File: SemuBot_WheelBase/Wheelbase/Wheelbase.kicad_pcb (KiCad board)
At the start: 2 copper layers, 100 x 80 mm, 120 parts, among them IC1 DRV8353FSRTAR, IC2 DRV8353FSRTAR, IC3 DRV8353FSRTAR, J1 10155435-00011LF, J10 B5B-XH-A_LF__SN_, J11 B5B-XH-A_LF__SN_, J12 B5B-XH-A_LF__SN_, J13 MTSW-104-09-L-S-400, J14 XT30PW-M, J15 MTSW-104-09-L-S-400, J2 MTSW-102-09-L-S-400, J3 MR30PW-M, J4 B5B-XH-A_LF__SN_, J5 B5B-XH-A_LF__SN_, J6 B5B-XH-A_LF__SN_, J7 MR30PW-M, J8 MR30PW-M, J9 DS1013-10SSIB1, Q1 AON7262E, Q10 AON7262E, Q11 AON7262E, Q12 AON7262E, Q13 AON7262E, Q14 AON7262E, Q15 AON7262E, Q19 AON7262E, Q2 AON7262E, Q20 AON7262E, Q21 AON7262E, Q3 AON7262E, Q4 AON7262E, Q5 AON7262E, Q6 AON7262E, Q7 AON7262E, Q8 AON7262E, Q9 AON7262E, U1 STM32F303RET6, U5 RT9013-33GB, Y2 X322516MLB4SI

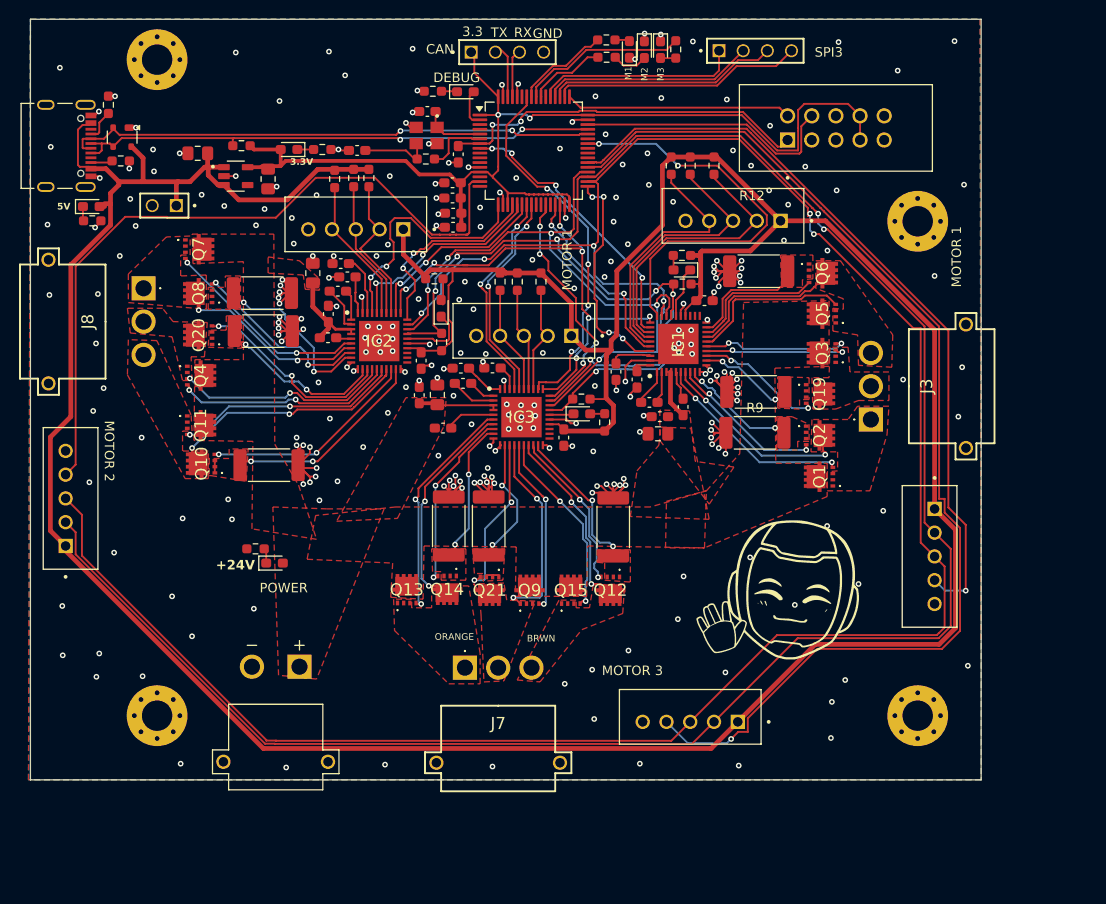
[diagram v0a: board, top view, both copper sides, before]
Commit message: Current sensing
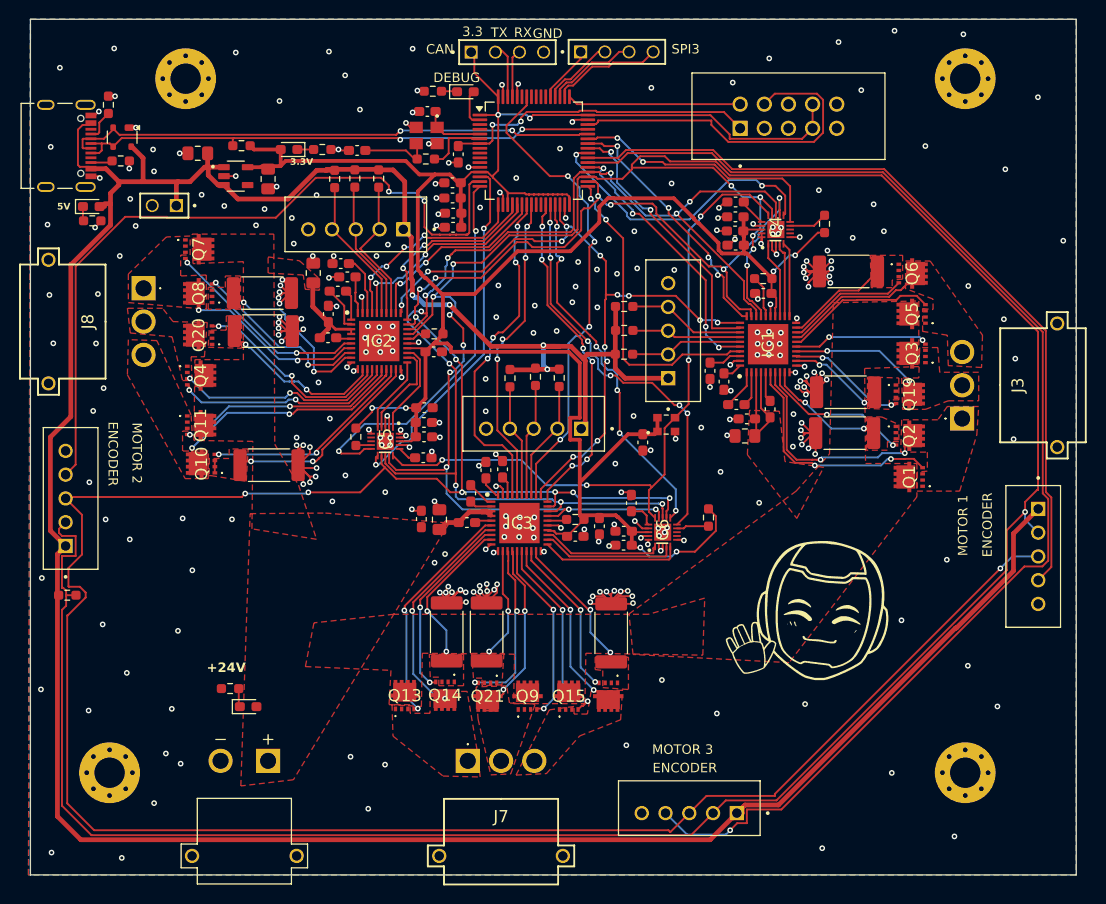
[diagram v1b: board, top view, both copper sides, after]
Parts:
- removed D10, D11, D12: red, LED_SMD:LED_0603_1608Metric_Pad1.05x0.95mm_HandSolder
- removed D4, D5, D6: LED, LED_SMD:LED_0603_1608Metric_Pad1.05x0.95mm_HandSolder
- removed the R21 at (162.3, 64.8)
- removed the R22 at (169.6, 63.9)
- removed R23, R24, R25: 3.3K, Resistor_SMD:R_0603_1608Metric_Pad0.98x0.95mm_HandSolder
- removed the R3 at (144.9, 94.7)
- added C16: 220nF, Capacitor_SMD:C_0603_1608Metric_Pad1.08x0.95mm_HandSolder, F.Cu at (175.8, 80.0)
- added C22: 220nF, Capacitor_SMD:C_0603_1608Metric_Pad1.08x0.95mm_HandSolder, F.Cu at (143.0, 106.9)
- added C34: 220nF, Capacitor_SMD:C_0603_1608Metric_Pad1.08x0.95mm_HandSolder, F.Cu at (164.9, 111.6)
- added C35: 100nF, Capacitor_SMD:C_0603_1608Metric_Pad1.08x0.95mm_HandSolder, F.Cu at (175.9, 84.5)
- added C36: 100nF, Capacitor_SMD:C_0603_1608Metric_Pad1.08x0.95mm_HandSolder, F.Cu at (143.1, 104.7)
- added C37: 100nF, Capacitor_SMD:C_0603_1608Metric_Pad1.08x0.95mm_HandSolder, F.Cu at (161.5, 114.1)
- added C38: 100nF, Capacitor_SMD:C_0603_1608Metric_Pad1.08x0.95mm_HandSolder, F.Cu at (175.8, 81.5)
- added C39: 100nF, Capacitor_SMD:C_0603_1608Metric_Pad1.08x0.95mm_HandSolder, F.Cu at (143.1, 103.2)
- added C40: 100nF, Capacitor_SMD:C_0603_1608Metric_Pad1.08x0.95mm_HandSolder, F.Cu at (164.1, 114.6)
- added C50: 100nF, Capacitor_SMD:C_0603_1608Metric_Pad1.08x0.95mm_HandSolder, F.Cu at (166.1, 105.3)
- added C51: 100nF, Capacitor_SMD:C_0603_1608Metric_Pad1.08x0.95mm_HandSolder, F.Cu at (175.8, 83.0)
- added C52: 100nF, Capacitor_SMD:C_0603_1608Metric_Pad1.08x0.95mm_HandSolder, F.Cu at (143.1, 101.6)
- added C53: 100nF, Capacitor_SMD:C_0603_1608Metric_Pad1.08x0.95mm_HandSolder, F.Cu at (164.1, 116.1)
- added IC4: ADS131M03IRUKT, ADS131M:QFN40P300X300X80-21N-D, F.Cu at (180.1, 82.9)
- added IC5: ADS131M03IRUKT, ADS131M:QFN40P300X300X80-21N-D, F.Cu at (139.0, 105.1)
- added IC6: ADS131M03IRUKT, ADS131M:QFN40P300X300X80-21N-D, F.Cu at (168.2, 114.7)
- added R32: 1.5K, Resistor_SMD:R_0603_1608Metric_Pad0.98x0.95mm_HandSolder, F.Cu at (164.1, 93.5)
- added R33: 1.5K, Resistor_SMD:R_0603_1608Metric_Pad0.98x0.95mm_HandSolder, F.Cu at (135.8, 77.5)
- added R34: 1.5K, Resistor_SMD:R_0603_1608Metric_Pad0.98x0.95mm_HandSolder, F.Cu at (154.8, 98.4)
- added R45: 3.3K, Resistor_SMD:R_0603_1608Metric_Pad0.98x0.95mm_HandSolder, F.Cu at (105.6, 121.3)
- added Y1: ECS-2520MVLC-081.92-CN-TR, ECS-2520:OSC_ECS-2520MVLC-081.92-CN-TR, F.Cu at (168.6, 103.4)
- moved H4 113.4 mm to (200.0, 140.0)
- moved H2 85.2 mm to (110.0, 140.0)
- moved H1 67.1 mm to (118.0, 67.0)
- moved R22 31.9 mm to (173.0, 113.2)
- moved R21 27.2 mm to (135.9, 104.7)
- moved R35 20.4 mm to (164.1, 96.0), turned to 180 degrees
- moved R29 17.6 mm to (164.1, 91.0), turned to 180 degrees
- moved H3 15.8 mm to (200.0, 67.0)
- moved R3 15.4 mm to (185.2, 82.3), turned to -90 degrees
- moved D7 15.4 mm to (124.6, 133.1)
- moved R18 14.9 mm to (122.7, 131.2)
- moved J15 14.6 mm to (163.4, 64.2)
- moved J4 13.6 mm to (169.3, 93.5), turned to -90 degrees
- moved C33 13.1 mm to (144.7, 113.4)
- moved C23 13.0 mm to (142.8, 113.3)
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- renumbered R33 to R21, R34 to R22, R32 to R3
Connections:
- C18 pad 1: +5V -> +3.3V
- C24 pad 1: +5V -> +3.3V
- C6 pad 1: +5V -> +3.3V
- IC1 pad 21: unconnected-(IC1-SOC-Pad21) -> /Motor_1/SOC
- IC1 pad 22: unconnected-(IC1-SOB-Pad22) -> /Motor_1/SOB
- IC1 pad 23: unconnected-(IC1-SOA-Pad23) -> /Motor_1/SOA
- IC1 pad 24: +5V -> +3.3V
- IC1 pad 26: Net-(D4-K) -> Net-(IC1-NFAULT)
- IC2 pad 21: unconnected-(IC2-SOC-Pad21) -> /Motor_2/SOC
- IC2 pad 22: unconnected-(IC2-SOB-Pad22) -> /Motor_2/SOB
- IC2 pad 23: unconnected-(IC2-SOA-Pad23) -> /Motor_2/SOA
- IC2 pad 24: +5V -> +3.3V
- IC2 pad 26: Net-(D5-K) -> Net-(IC2-NFAULT)
- IC3 pad 21: unconnected-(IC3-SOC-Pad21) -> /Motor_3/SOC
- IC3 pad 22: unconnected-(IC3-SOB-Pad22) -> /Motor_3/SOB
- IC3 pad 23: unconnected-(IC3-SOA-Pad23) -> /Motor_3/SOA
- IC3 pad 24: +5V -> +3.3V
- IC3 pad 26: Net-(D6-K) -> Net-(IC3-NFAULT)
- J4 pad 2: /Motor_1/HAL_1 -> /Motor_1/HAL_3
- J4 pad 4: /Motor_1/HAL_3 -> /Motor_1/HAL_1
- R21 pad 1: /Motor_2/HAL_2 -> Net-(IC5-~{SYNC_}/_~{RESET})
- R21 pad 2: +5V -> +3.3V
- R22 pad 1: /Motor_3/HAL_2 -> Net-(IC6-~{SYNC_}/_~{RESET})
- R22 pad 2: +5V -> +3.3V
- R3 pad 1: /Motor_1/HAL_2 -> Net-(IC4-~{SYNC_}/_~{RESET})
- R3 pad 2: +5V -> +3.3V
- R4 pad 1: Net-(D4-A) -> Net-(IC1-NFAULT)
- R4 pad 2: +5V -> +3.3V
- R7 pad 1: Net-(D5-A) -> Net-(IC2-NFAULT)
- R7 pad 2: +5V -> +3.3V
- R8 pad 1: Net-(D6-A) -> Net-(IC3-NFAULT)
- R8 pad 2: +5V -> +3.3V
- U1 pad 14: unconnected-(U1-PA0-Pad14) -> /motor2_DRDY
- U1 pad 16: unconnected-(U1-PA2-Pad16) -> /motor2_adc
- U1 pad 28: unconnected-(U1-PB2-Pad28) -> /motor3_adc
- U1 pad 29: /MOTOR1_DIR -> /motor3_DRDY
- U1 pad 37: /CS_ENC_3 -> /MOTOR1_DIR
- U1 pad 38: /CS_ENC_1 -> /CS_ENC_3
- U1 pad 39: unconnected-(U1-PC8-Pad39) -> /CS_ENC_1
- U1 pad 40: unconnected-(U1-PC9-Pad40) -> /motor1_DRDY
- U1 pad 41: unconnected-(U1-PA8-Pad41) -> /MOTOR1_PWM
- U1 pad 43: unconnected-(U1-PA10-Pad43) -> /motor1_adc
- U1 pad 55: /motor2_led -> unconnected-(U1-PB3-Pad55)
- U1 pad 56: /motor3_led -> unconnected-(U1-PB4-Pad56)
- U1 pad 57: /motor1_led -> unconnected-(U1-PB5-Pad57)
- U1 pad 8: /MOTOR1_PWM -> unconnected-(U1-PC0-Pad8)
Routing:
- net +3.3V: track 113.7 -> 281.9 mm, vias 2 -> 8
- net /SPI_DATA: track 264.0 -> 352.6 mm, vias 8 -> 14
- net /adc_CLK: track 0.00 -> 72.4 mm, vias 0 -> 4
- net /SPI_MOSI: track 69.5 -> 128.7 mm, vias 5 -> 10
- net +5V: track 374.4 -> 316.7 mm, vias 0 -> 4
- net /SPI_CLK: track 256.9 -> 311.3 mm, vias 7 -> 15
- net /motor3_adc: track 0.00 -> 43.2 mm, vias 0 -> 6
- net /motor2_adc: track 0.00 -> 40.6 mm, vias 0 -> 2
- net /motor3_DRDY: track 0.00 -> 39.4 mm, vias 0 -> 6
- net /motor2_DRDY: track 0.00 -> 37.8 mm, vias 0 -> 2
- net /motor1_DRDY: track 0.00 -> 31.3 mm, vias 0 -> 2
- net /motor1_adc: track 0.00 -> 27.2 mm, vias 0 -> 2
- net GND: track 181.2 -> 207.7 mm, vias 266 -> 303
- net /ENABLE: track 55.2 -> 74.8 mm, vias 7 -> 13
- net /motor3_led: track 17.8 -> 0.00 mm
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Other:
- board size 100 x 80 mm -> 110 x 90 mm
- board text added: "ENCODER"
- board text removed: "BRWN"
- board text removed: "M1"
- board text removed: "M2"
- board text removed: "M3"
- board text removed: "ORANGE"
- board text removed: "POWER"
